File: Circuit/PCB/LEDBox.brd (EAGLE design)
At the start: 28 x 28 mm, 17 parts, among them SW6 B3F-1000

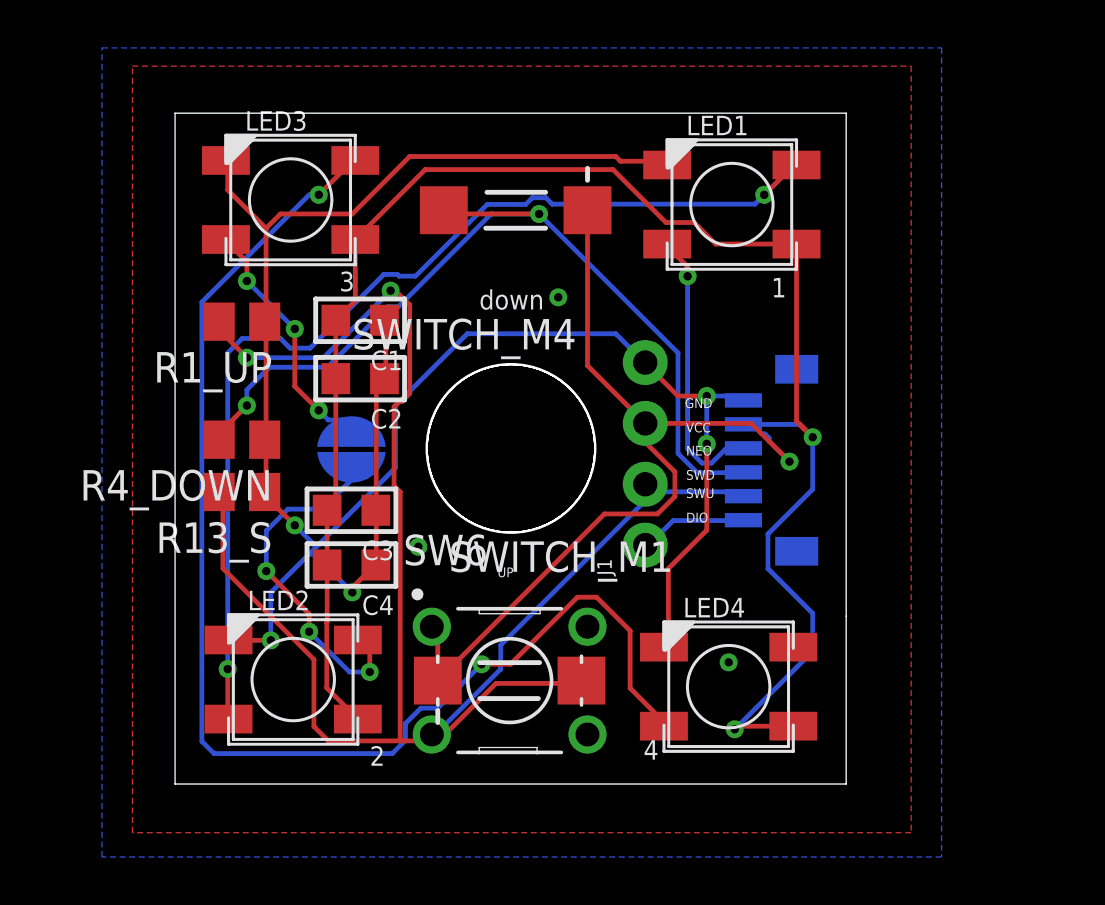
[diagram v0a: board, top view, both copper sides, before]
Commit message: merge
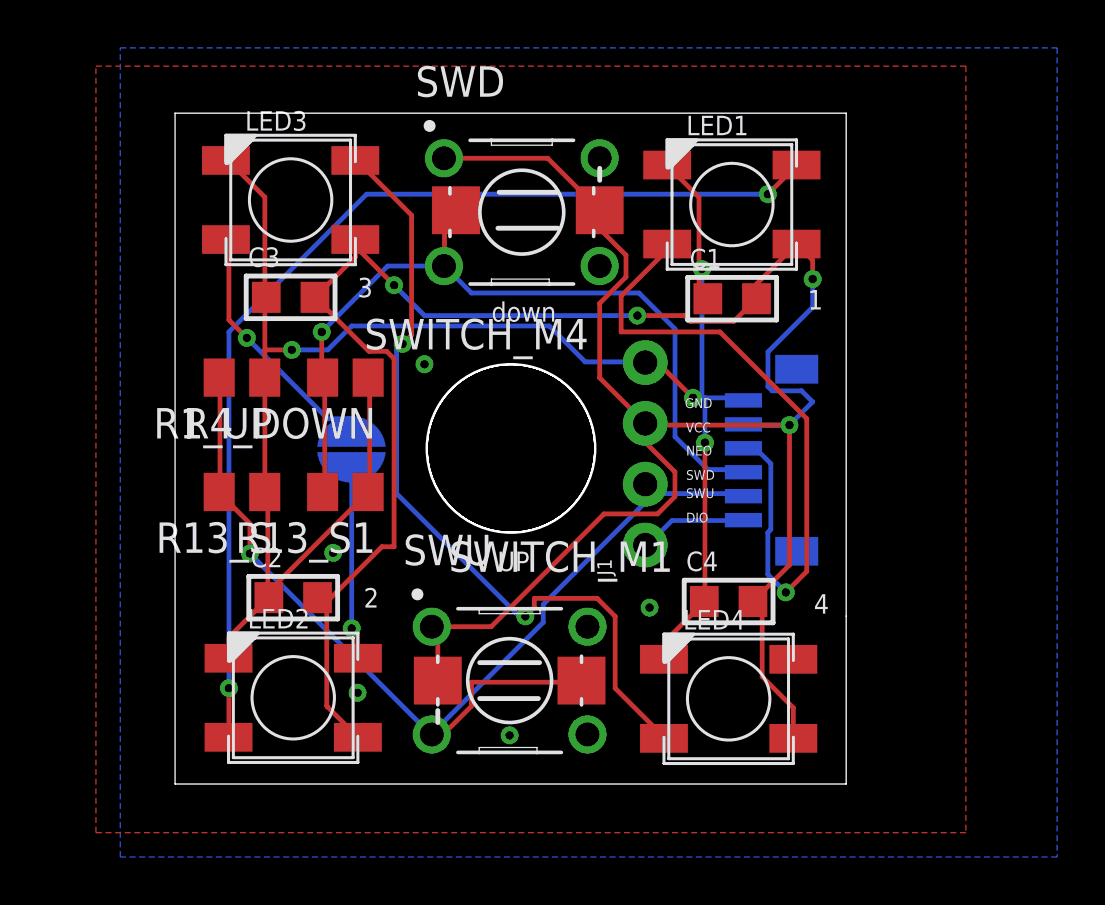
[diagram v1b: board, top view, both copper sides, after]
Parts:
- added R13_S1: 10K, resistor:M0805
- added SWD: B3F-1000, Switch:B3F-1000
- moved C4 15.8 mm to (23.1, 7.62), turned to 0 degrees
- moved C1 15.6 mm to (23.3, 20.3), turned to 0 degrees
- moved C2 9.56 mm to (4.93, 7.78), turned to 0 degrees
- moved C3 9.25 mm to (4.83, 20.3), turned to 0 degrees
- moved R4_DOWN 5.04 mm to (7.11, 17.0)
- moved R1_UP 2.34 mm to (2.79, 17.0)
- moved LED2 0.76 mm to (4.93, 3.60)
- moved SWITCH_M4 0.51 mm to (14.7, 24.0)
- moved LED4 0.51 mm to (23.1, 3.56)
- renumbered SW6 to SWU
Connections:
- net GND: now also R13_S1.1
- net SWD_IN: now also R13_S1.2, SWD.3
- net VCC: now also SWD.1
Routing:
- net SWU_IN: track 71.6 -> 45.1 mm, vias 2 -> 1
- net N$6: track 53.7 -> 33.2 mm
- net NEO_IN: track 11.7 -> 28.5 mm
- net GND: track 92.4 -> 78.8 mm, vias 8 -> 9
- net VCC: track 109.7 -> 116.7 mm, vias 3 -> 4
- net N$2: track 14.2 -> 7.56 mm, vias 3 -> 1
- net SWD_IN: track 37.4 -> 34.3 mm, vias 2 -> 1
- net N$1: track 42.9 -> 43.5 mm
- net N$4: track 10.3 -> 10.2 mm, vias 3 -> 1
